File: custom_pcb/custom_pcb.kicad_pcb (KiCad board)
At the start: 2 copper layers, 285 x 152 mm, 316 parts, among them J1 USB_mini_micro_B, K0 KEYSW, K1 KEYSW, K10 KEYSW, K11 KEYSW, K12 KEYSW, K13 KEYSW, K14 KEYSW, K15 KEYSW, K16 KEYSW, K17 KEYSW, K18 KEYSW, K19 KEYSW, K2 KEYSW, K20 KEYSW, K21 KEYSW, K22 KEYSW, K23 KEYSW, K24 KEYSW, K25 KEYSW, K26 KEYSW, K27 KEYSW, K28 KEYSW, K29 KEYSW, K3 KEYSW, K30 KEYSW, K31 KEYSW, K32 KEYSW, K33 KEYSW, K34 KEYSW, K35 KEYSW, K36 KEYSW, K37 KEYSW, K38 KEYSW, K39 KEYSW, K4 KEYSW, K40 KEYSW, K41 KEYSW, K42 KEYSW, K43 KEYSW, K44 KEYSW, K45 KEYSW, K46 KEYSW, K47 KEYSW, K48 KEYSW, K49 KEYSW, K5 KEYSW, K50 KEYSW, K51 KEYSW, K52 KEYSW, K53 KEYSW, K54 KEYSW, K55 KEYSW, K56 KEYSW, K57 KEYSW, K58 KEYSW, K59 KEYSW, K6 KEYSW, K60 KEYSW, K63 KEYSW, K64 KEYSW, K65 KEYSW, K66 KEYSW, K67 KEYSW, K68 KEYSW, K69 KEYSW, K7 KEYSW, K70 KEYSW, K71 KEYSW, K72 KEYSW, K73 KEYSW, K74 KEYSW, K75 KEYSW, K76 KEYSW, K77 KEYSW, K78 KEYSW, K79 KEYSW, K8 KEYSW, K80 KEYSW, K81 KEYSW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

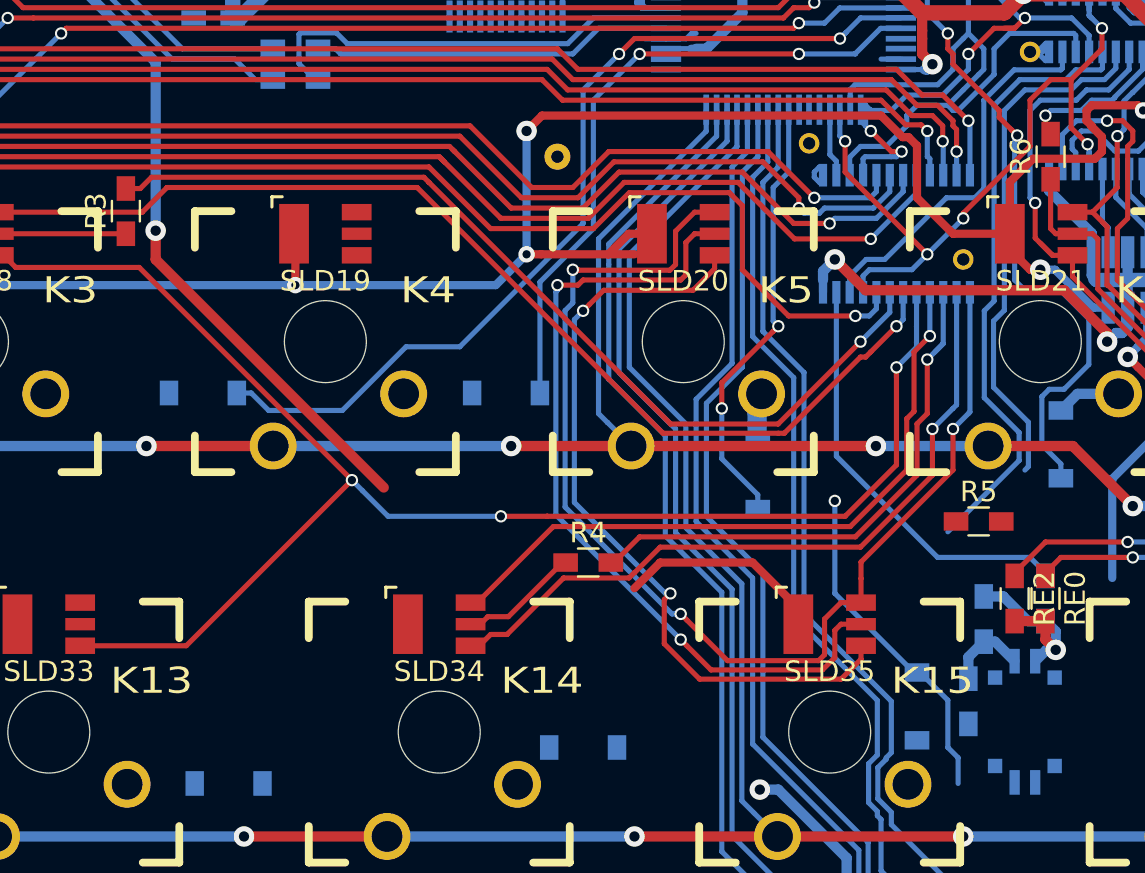
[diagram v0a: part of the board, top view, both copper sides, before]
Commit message: tweaks
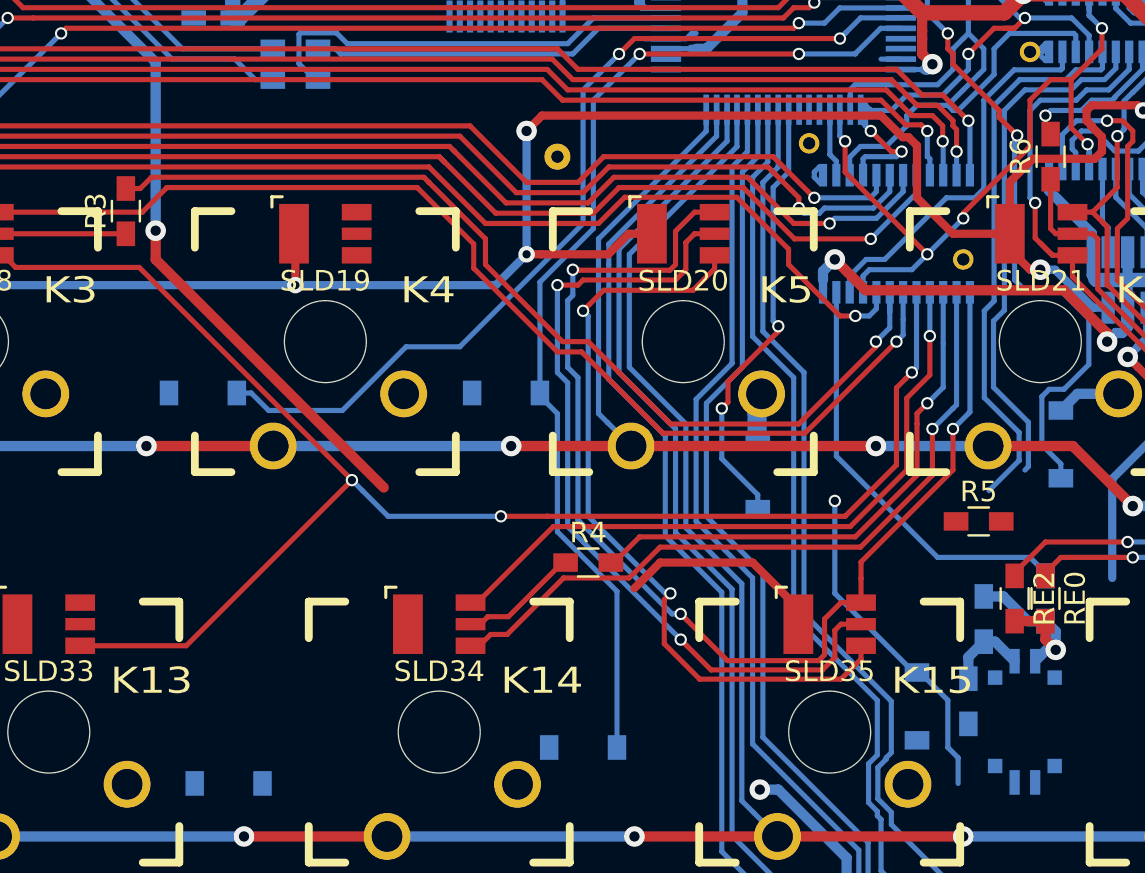
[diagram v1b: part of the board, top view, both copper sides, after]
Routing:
- net c4: track 31.8 -> 50.6 mm
- net green5: track 67.7 -> 64.6 mm
- net Net-(LC1-Pad19): track 45.6 -> 47.9 mm
- net green2: track 69.5 -> 67.7 mm
- net anode0: track 174.7 -> 173.4 mm
- net blue3: track 53.1 -> 54.2 mm
- net Net-(LC1-Pad15): track 26.7 -> 26.1 mm
